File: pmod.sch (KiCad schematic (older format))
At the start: 13 parts, among them J6 PMOD, U10 AP7381-33SA, U11 TXS0108EPW

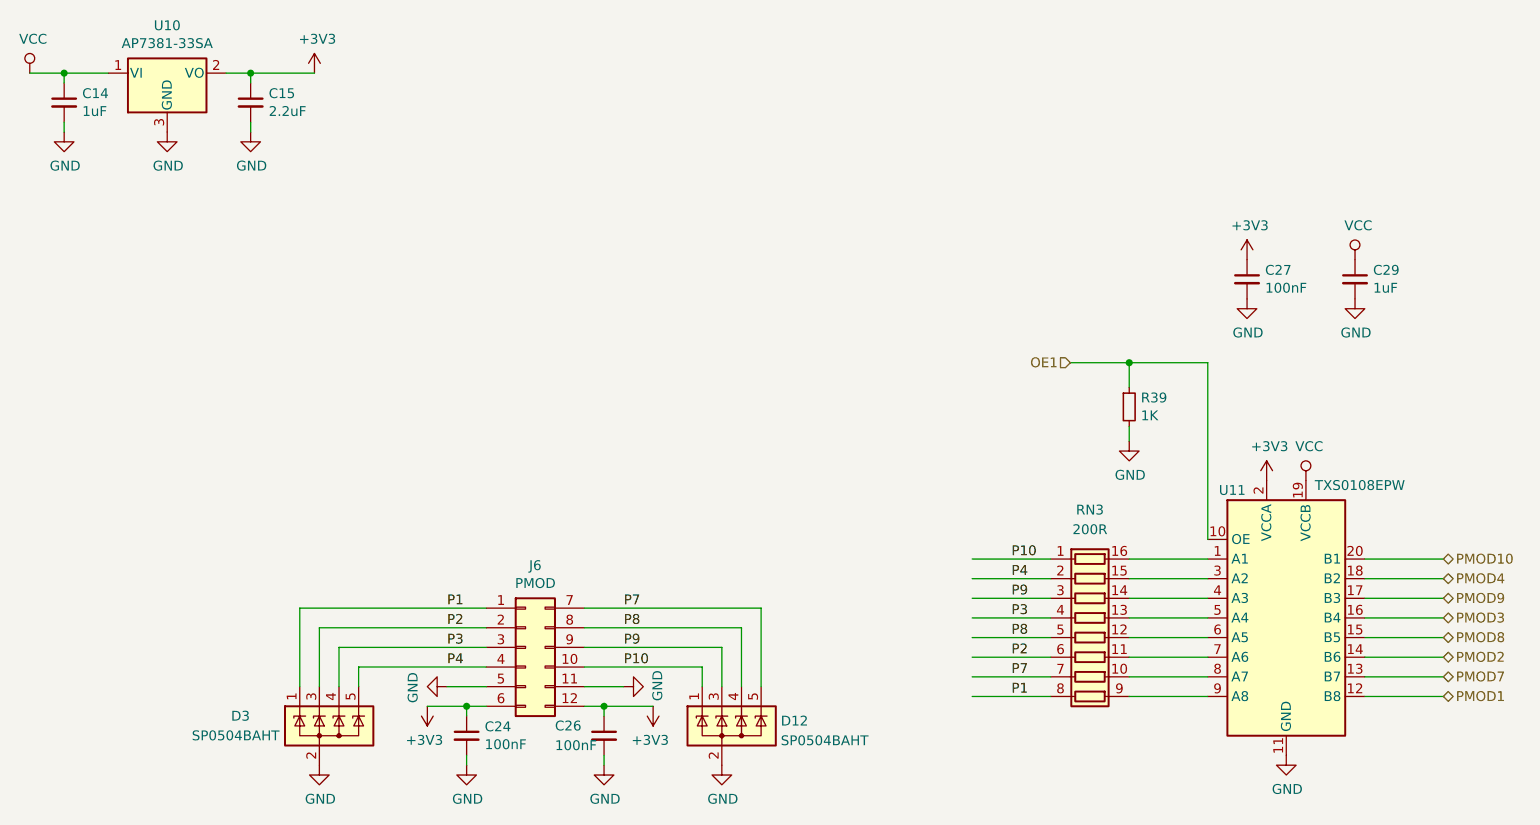
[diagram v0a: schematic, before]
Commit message: lots of fixes
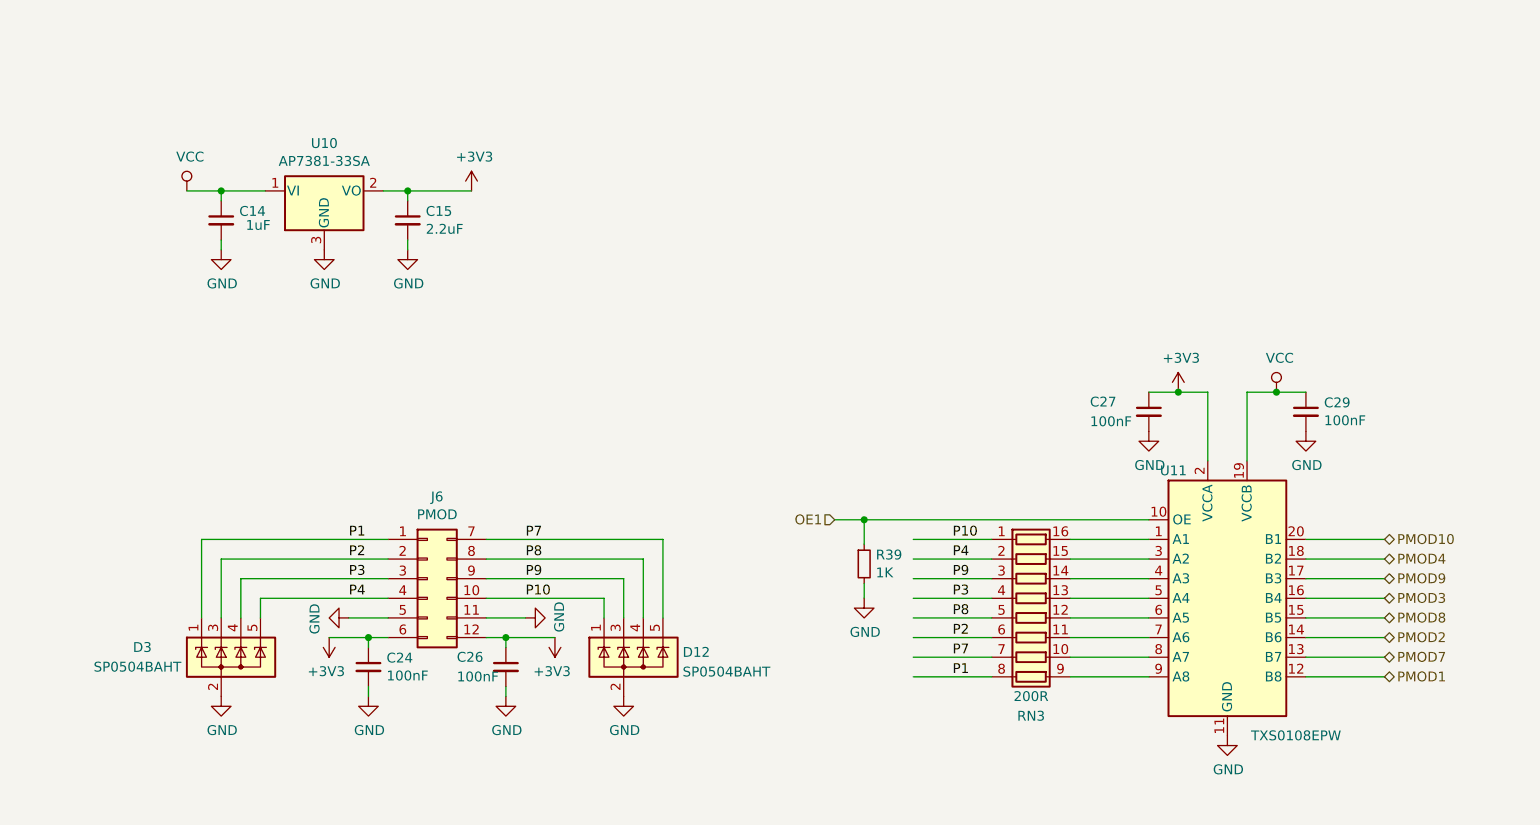
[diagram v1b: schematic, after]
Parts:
- C29: value 1uF -> 100nF
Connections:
- wire segments 63 -> 68
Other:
- moved on the sheet: C14, C15, C24, C26, C27, C29, D12, D3, J6, R39, RN3, U10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
